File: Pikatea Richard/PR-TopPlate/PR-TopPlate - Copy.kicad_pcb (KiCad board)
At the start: 2 copper layers, 66 x 138.1 mm, 7 parts, among them SW1 Rotary_Encoder_Switch, SW2 Rotary_Encoder_Switch

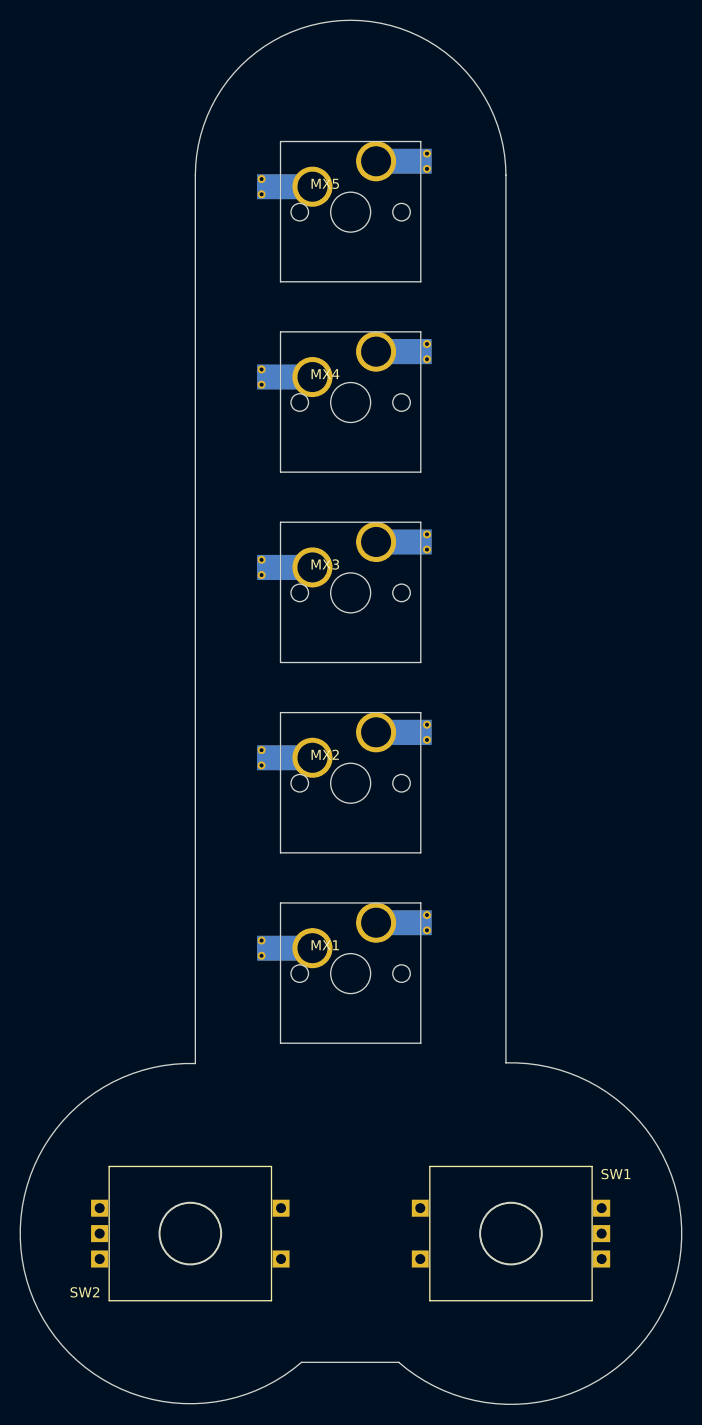
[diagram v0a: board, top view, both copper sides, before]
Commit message: updated footprints added gerbers
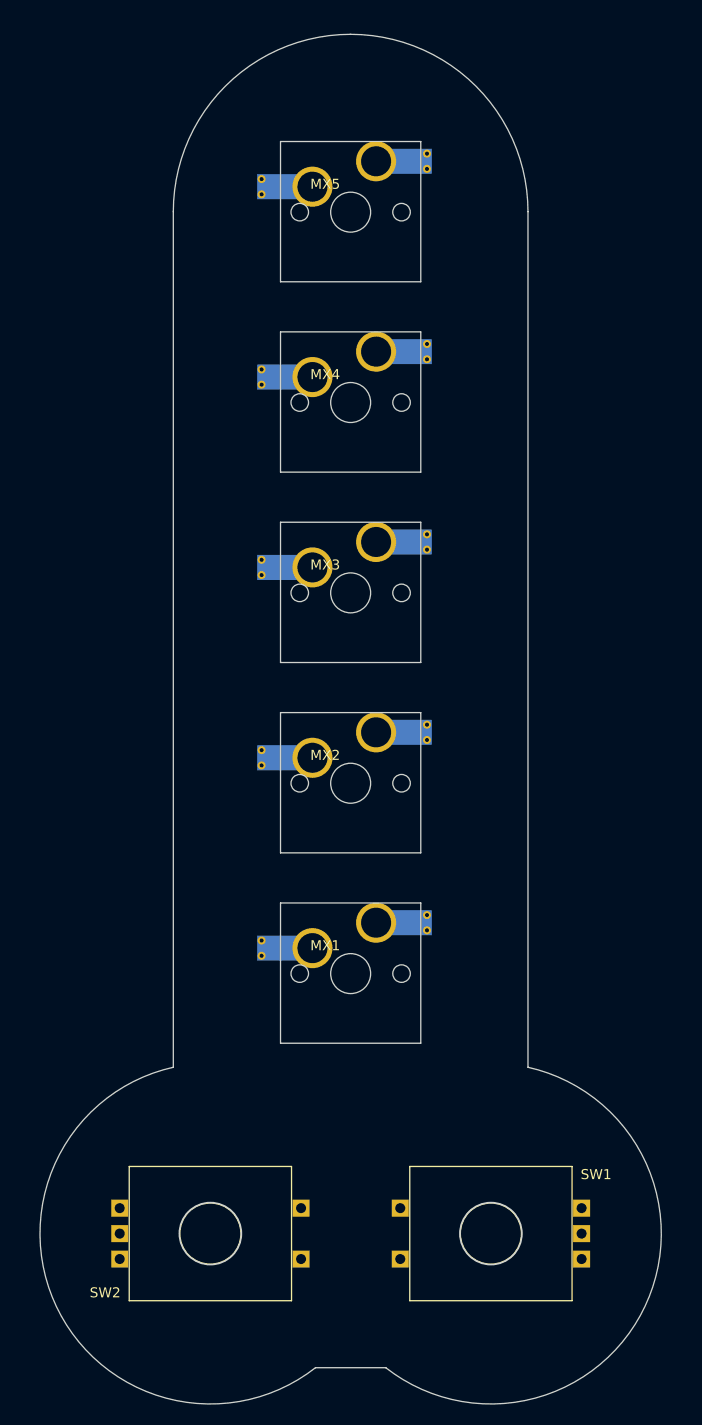
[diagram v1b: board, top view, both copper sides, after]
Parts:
- moved SW1 2.00 mm to (153.0, 100.0)
- moved SW2 2.00 mm to (125.0, 100.0)
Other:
- board size 66 x 138.1 mm -> 62 x 136.7 mm
